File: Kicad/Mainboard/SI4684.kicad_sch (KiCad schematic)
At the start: 89 parts, among them J1 DC IN, J2 Ant, J3 Headphones, J4 FRONT-PCB, J5 AUDIO, U1 MIC5504-1.8YM5, U2 LM2596T-5, U3 SI4684-A10-GM, U4 LM1117T-3.3, U5 TPA6130A2RTJTG4, U6 NE5532, X1 19.2MHz

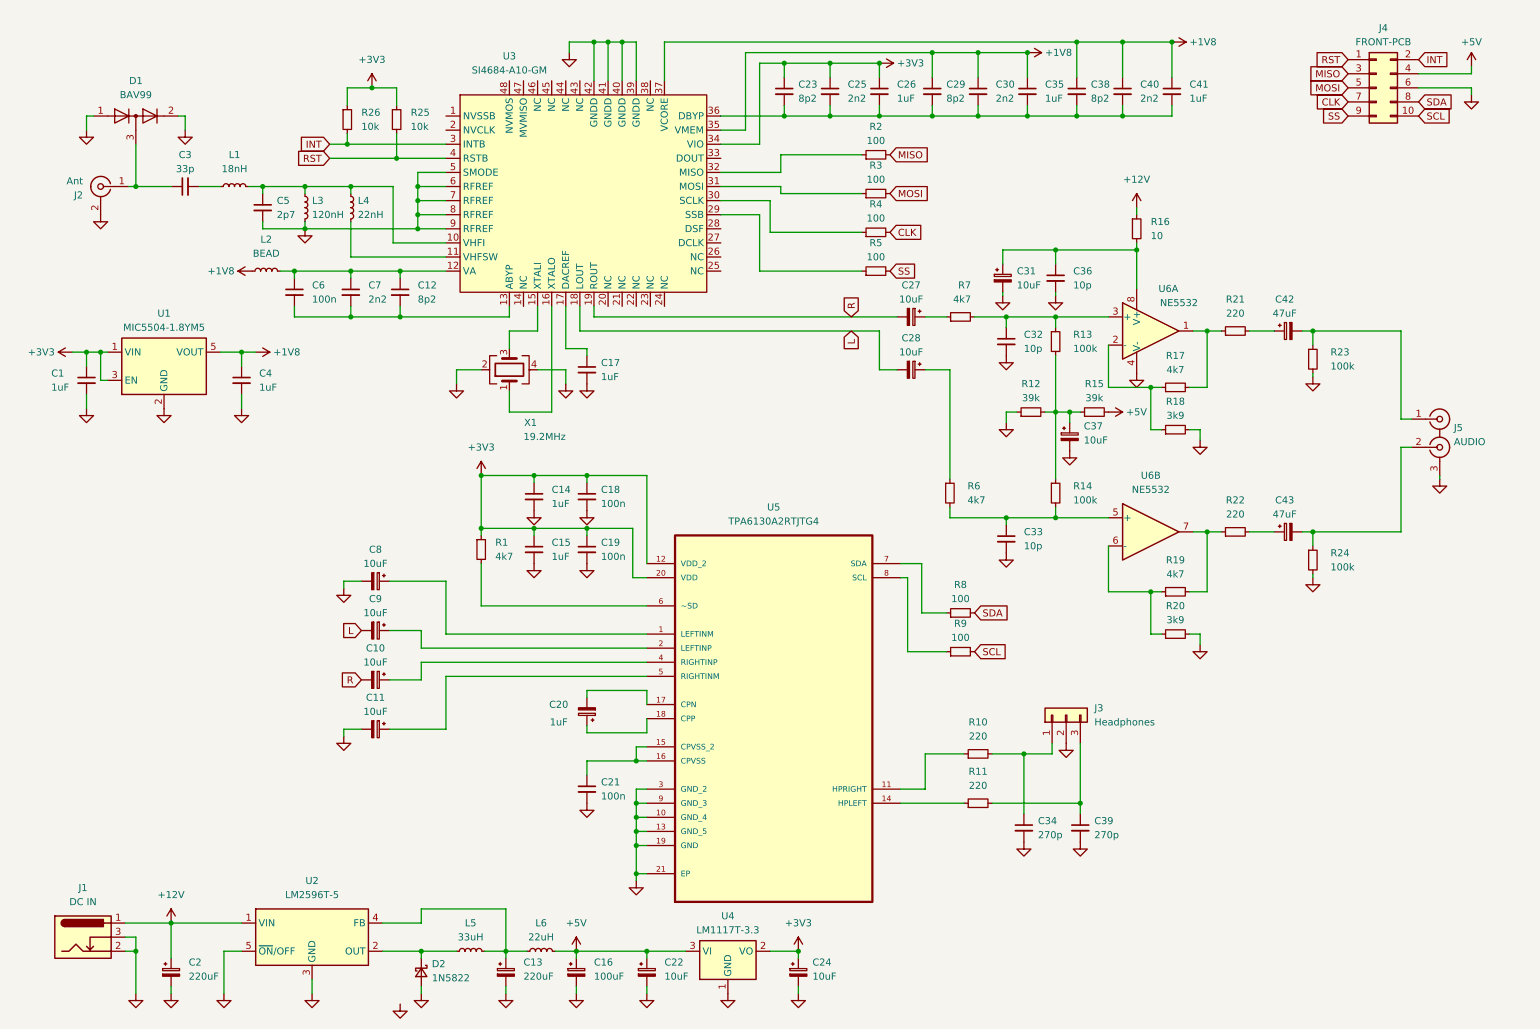
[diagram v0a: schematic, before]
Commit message: Add files via upload
work in progress. not finished
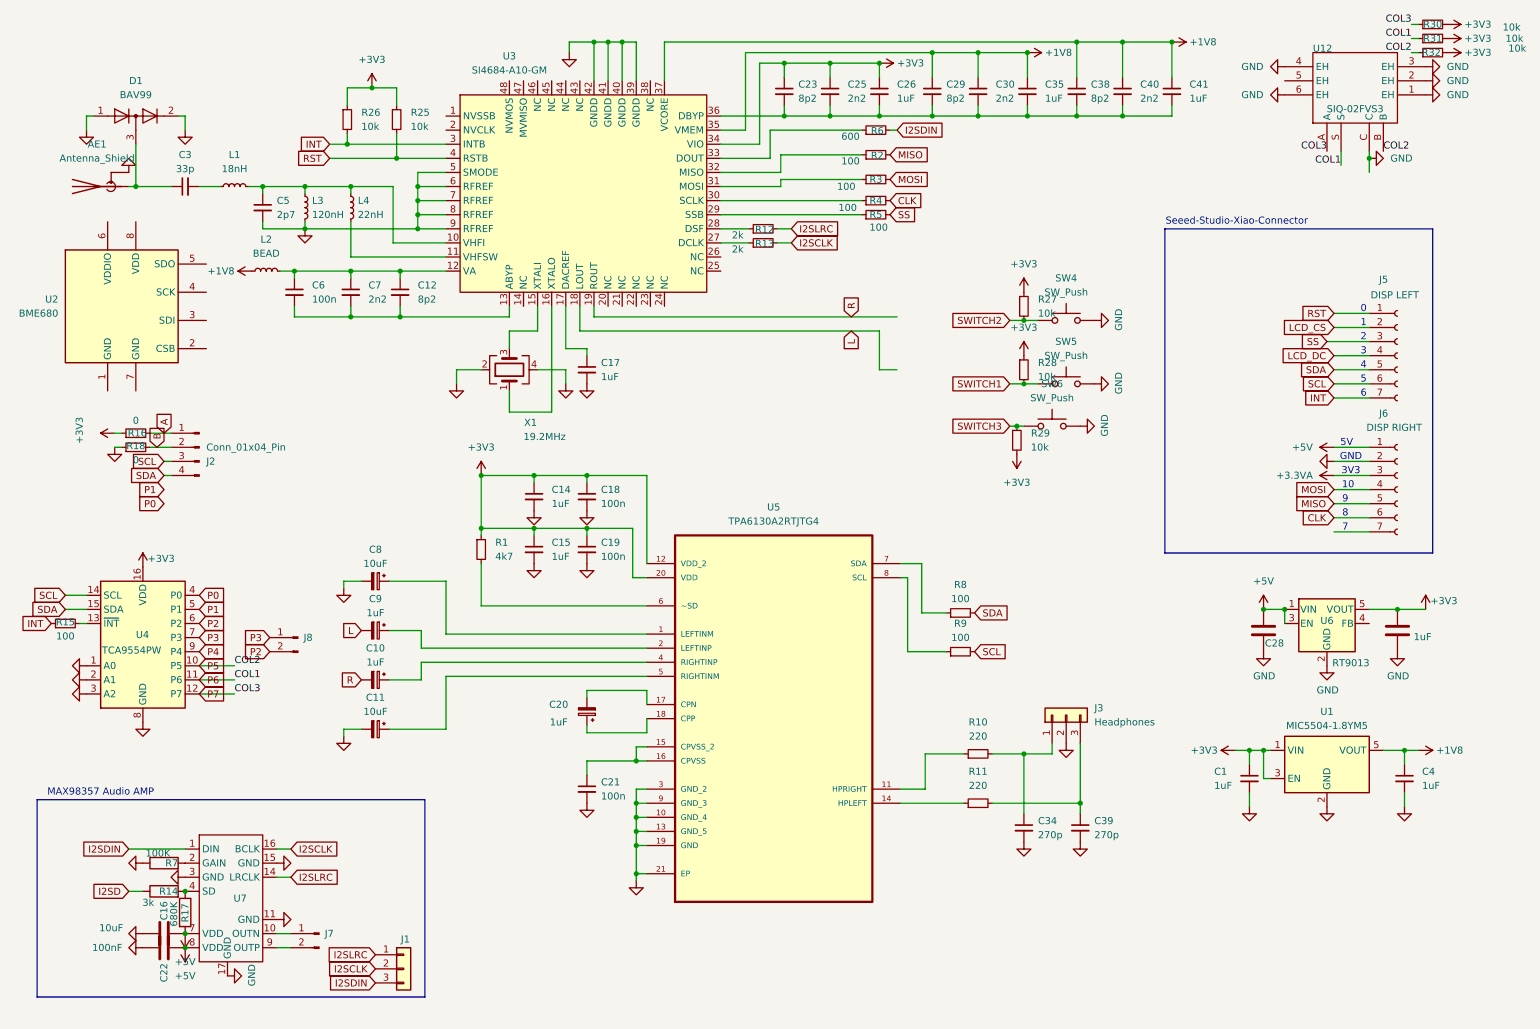
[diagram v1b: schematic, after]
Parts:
- removed C13, C2: 220uF, Capacitor_THT:CP_Radial_D10.0mm_P3.50mm, symbol Device:C_Polarized_Small
- removed C16: 100uF, Capacitor_THT:CP_Radial_D10.0mm_P3.50mm, symbol Device:C_Polarized_Small
- removed C22, C24, C27, C28, C31, C37: 10uF, Capacitor_THT:CP_Radial_D5.0mm_P2.00mm, symbol Device:C_Polarized_Small
- removed C32, C33, C36: 10p, Capacitor_THT:C_Disc_D3.0mm_W2.0mm_P2.50mm, symbol Device:C_Small
- removed C42, C43: 47uF, Capacitor_THT:CP_Radial_D5.0mm_P2.00mm, symbol Device:C_Polarized_Small
- removed D2: 1N5822, Diode_THT:D_DO-201_P12.70mm_Horizontal, symbol Device:D_Schottky_Small
- removed J1: DC IN, Connector_BarrelJack:BarrelJack_Horizontal, symbol Connector:Barrel_Jack_Switch
- removed J2: Ant, Connector_Coaxial:SMA_Amphenol_132134-16_Vertical, symbol Connector:Conn_Coaxial
- removed J4: FRONT-PCB, Connector_IDC:IDC-Header_2x05_P2.54mm_Vertical, symbol Connector_Generic:Conn_02x05_Odd_Even
- removed J5: AUDIO, Library:FC68405_cinch, symbol Connector:Conn_Coaxial_x2
- removed L5: 33uH, Inductor_THT:L_Radial_D7.2mm_P3.00mm_Murata_1700, symbol Device:L_Small
- removed L6: 22uH, Inductor_THT:L_Radial_D7.2mm_P3.00mm_Murata_1700, symbol Device:L_Small
- removed R14, R23, R24: 100k, Resistor_THT:R_Axial_DIN0207_L6.3mm_D2.5mm_P10.16mm_Horizontal, symbol Device:R_Small
- removed R17, R19, R7: 4k7, Resistor_THT:R_Axial_DIN0207_L6.3mm_D2.5mm_P10.16mm_Horizontal, symbol Device:R_Small
- removed R20: 3k9, Resistor_THT:R_Axial_DIN0207_L6.3mm_D2.5mm_P10.16mm_Horizontal, symbol Device:R_Small
- removed R21, R22: 220, Resistor_THT:R_Axial_DIN0207_L6.3mm_D2.5mm_P10.16mm_Horizontal, symbol Device:R_Small
- removed U2: LM2596T-5, Package_TO_SOT_THT:TO-220-5_Vertical, symbol Regulator_Switching:LM2596T-5
- removed U4: LM1117T-3.3, Package_TO_SOT_THT:TO-220-3_Vertical, symbol Regulator_Linear:LM1117T-3.3
- removed U6: NE5532, Package_DIP:DIP-8_W7.62mm_LongPads, symbol Amplifier_Operational:NE5532
- added AE1: Antenna_Shield, Connector_Coaxial:SMA_Samtec_SMA-J-P-H-ST-EM1_EdgeMount, symbol Device:Antenna_Shield
- added C16: 10uF, Capacitor_SMD:C_0805_2012Metric_Pad1.18x1.45mm_HandSolder, symbol Device:C
- added C22: 100nF, Capacitor_SMD:C_0805_2012Metric_Pad1.18x1.45mm_HandSolder, symbol Device:C
- added C28, C31: 1uF, Capacitor_SMD:C_0805_2012Metric_Pad1.18x1.45mm_HandSolder, symbol Device:C
- added J1: Conn_01x03, Connector_PinHeader_2.54mm:PinHeader_1x03_P2.54mm_Vertical, symbol Connector_Generic:Conn_01x03
- added J2: Conn_01x04_Pin, Connector_PinHeader_2.54mm:PinHeader_1x04_P2.54mm_Vertical, symbol Connector:Conn_01x04_Pin
- added J5: DISP LEFT, Connector_PinHeader_2.54mm:PinHeader_1x07_P2.54mm_Vertical, symbol Connector:Conn_01x07_Socket
- added J6: DISP RIGHT, Connector_PinHeader_2.54mm:PinHeader_1x07_P2.54mm_Vertical, symbol Connector:Conn_01x07_Socket
- added J7, J8: Conn_01x02_Pin, Connector_PinHeader_2.54mm:PinHeader_1x02_P2.54mm_Vertical, symbol Connector:Conn_01x02_Pin
- added R14: 3k, Resistor_SMD:R_0805_2012Metric_Pad1.20x1.40mm_HandSolder, symbol Device:R
- added R17: 680K, Resistor_SMD:R_0805_2012Metric_Pad1.20x1.40mm_HandSolder, symbol Device:R
- added R27, R28, R29: 10k, Resistor_SMD:R_0805_2012Metric_Pad1.20x1.40mm_HandSolder, symbol Device:R_Small
- added R30, R31, R32: 10k, Resistor_SMD:R_0603_1608Metric_Pad0.98x0.95mm_HandSolder, symbol Device:R_Small
- added R7: 100K, Resistor_SMD:R_0805_2012Metric_Pad1.20x1.40mm_HandSolder, symbol Device:R
- added SW4, SW5, SW6: SW_Push, tp4056:SW_SPST_CK_KMS2xxGP, symbol Switch:SW_Push
- added U12: SIQ-02FVS3, tp4056:SW-SMD_SIQ-02FVS3_1, symbol ProPrj_tes-easyedapro:SIQ-02FVS3
- added U2: BME680, Package_LGA:Bosch_LGA-8_3x3mm_P0.8mm_ClockwisePinNumbering, symbol Sensor:BME680
- added U4: TCA9554PW, Package_SO:TSSOP-16_4.4x5mm_P0.65mm, symbol Interface_Expansion:TCA9554PW
- added U6: RT9013, Package_TO_SOT_SMD:SOT-23-5, symbol Regulator_Linear:TPS72201
- added U7: ~, tp4056:TQFN-16_L3.0-W3.0-P0.50-BL-EP1.5, symbol MAX98357AETE+T:MAX98357A
- C10, C9: value 10uF -> 1uF; footprint Capacitor_THT:CP_Radial_D5.0mm_P2.00mm -> Capacitor_SMD:C_0805_2012Metric_Pad1.18x1.45mm_HandSolder
- C11, C8: footprint Capacitor_THT:CP_Radial_D5.0mm_P2.00mm -> Capacitor_SMD:C_0805_2012Metric_Pad1.18x1.45mm_HandSolder
- C20: footprint Capacitor_THT:CP_Radial_D5.0mm_P2.00mm -> Capacitor_SMD:C_0603_1608Metric
- C5: footprint Capacitor_SMD:C_0603_1608Metric -> Capacitor_SMD:C_0603_1608Metric_Pad1.08x0.95mm_HandSolder
- D1: footprint Package_TO_SOT_SMD:SOT-23 -> Package_TO_SOT_SMD:SOT-23W
- L1, L3, L4: footprint Inductor_SMD:L_0603_1608Metric -> Inductor_SMD:L_0603_1608Metric_Pad1.05x0.95mm_HandSolder
- R12: value 39k -> 2k; footprint Resistor_THT:R_Axial_DIN0207_L6.3mm_D2.5mm_P10.16mm_Horizontal -> Resistor_SMD:R_0603_1608Metric
- R13: value 100k -> 2k; footprint Resistor_THT:R_Axial_DIN0207_L6.3mm_D2.5mm_P10.16mm_Horizontal -> Resistor_SMD:R_0603_1608Metric
- R15: value 39k -> 100; footprint Resistor_THT:R_Axial_DIN0207_L6.3mm_D2.5mm_P10.16mm_Horizontal -> Resistor_SMD:R_0603_1608Metric
- R16: value 10 -> 0; footprint Resistor_THT:R_Axial_DIN0207_L6.3mm_D2.5mm_P10.16mm_Horizontal -> Resistor_SMD:R_0603_1608Metric
- R18: value 3k9 -> 0; footprint Resistor_THT:R_Axial_DIN0207_L6.3mm_D2.5mm_P10.16mm_Horizontal -> Resistor_SMD:R_0603_1608Metric
- R6: value 4k7 -> 600; footprint Resistor_THT:R_Axial_DIN0207_L6.3mm_D2.5mm_P10.16mm_Horizontal -> Resistor_SMD:R_0603_1608Metric
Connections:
- net +12V is gone; now on net +3V3: R16.1
- net +3V3: now also C31.2, R27.1, R28.1, R29.2, R30.2, R31.2, R32.2, U4.16 (VDD), U6.5 (VOUT)
- net +5V: now also C16.1, C22.1, C28.2, J6.1 (Pin_1), R17.2, U6.1 (VIN), U6.3 (EN), U7.7 (VDD), U7.8 (VDD); no longer R15.2
- net CLK: now also J6.6 (Pin_6)
- net GND: now also R18.1, AE1.2 (Shield), C16.2, C22.2, C28.1, C31.1, J6.2 (Pin_2), R7.1, SW4.2, SW5.1, SW6.1, U12.1 (EH), U12.2 (EH), U12.3 (EH), U12.4 (EH), U12.6 (EH), U12.C, U4.1 (A0), U4.2 (A1), U4.3 (A2), U4.8 (GND), U6.2 (GND), U7.11 (GND), U7.15 (GND), U7.17 (GND), U7.3 (GND); no longer R12.1, R18.2
- net INT: now also R15.1, J5.7 (Pin_7)
- net MISO: now also J6.5 (Pin_5)
- net MOSI: now also J6.4 (Pin_4)
- net RST: now also J5.1 (Pin_1)
- net SCL: now also J2.3 (Pin_3), J5.6 (Pin_6), U4.14 (SCL)
- net SDA: now also J2.4 (Pin_4), J5.5 (Pin_5), U4.15 (SDA)
- net SS: now also J5.3 (Pin_3)
- net at C3.1, D1.3 (K): now also AE1.1 (A)
- net at R6.1: now also U3.33 (DOUT)
- net I2SDIN: now reaches R6.2
- net I2SDIN: now also J1.3 (Pin_3), U7.1 (DIN)
- net A: now reaches R16.2
- net A: now also J2.1 (Pin_1)
- net at R13.1: now also U3.27 (DCLK)
- net at U3.28 (DSF): now also R12.1
- new net: R15.2, U4.13 (~{INT})
- new net: R7.2, U7.2 (GAIN)
- new net: R14.2, R17.1, U7.4 (SD)
- new net: J7.1 (Pin_1), U7.10 (OUTN)
- new net: J7.2 (Pin_2), U7.9 (OUTP)
- new net +3.3VA: J6.3 (Pin_3)
- new net B: J2.2 (Pin_2), R18.2
- new net I2SCLK: J1.2 (Pin_2), R13.2, U7.16 (BCLK)
- new net I2SD: R14.1
- new net I2SLRC: J1.1 (Pin_1), R12.2, U7.14 (LRCLK)
- new net LCD_CS: J5.2 (Pin_2)
- new net LCD_DC: J5.4 (Pin_4)
- new net P0: U4.4 (P0)
- new net P1: U4.5 (P1)
- new net P2: J8.2 (Pin_2), U4.6 (P2)
- new net P3: J8.1 (Pin_1), U4.7 (P3)
- new net P4: U4.9 (P4)
- new net P5: R32.1, U12.B, U4.10 (P5)
- new net P6: R31.1, U12.S, U4.11 (P6)
- new net P7: R30.1, U12.A, U4.12 (P7)
- new net SWITCH1: R28.2, SW5.2
- new net SWITCH2: R27.2, SW4.1
- new net SWITCH3: R29.1, SW6.2
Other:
- note added: "0"
- note added: "1"
- note added: "10"
- note added: "2"
- note added: "3"
- note added: "3V3"
- note added: "4"
- note added: "5"
- note added: "5V"
- note added: "6"
- note added: "7"
- note added: "8"
- note added: "9"
- note added: "GND"
- note added: "MAX98357 Audio AMP"
- note added: "Seeed-Studio-Xiao-Connector"
- moved on the sheet: C1, C4, R3, R4, R5, U1
